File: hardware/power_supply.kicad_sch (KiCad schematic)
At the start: 13 parts, among them U103 K78L15-1000R3, U105 AMS1117-5, U106 AMS1117-3.3

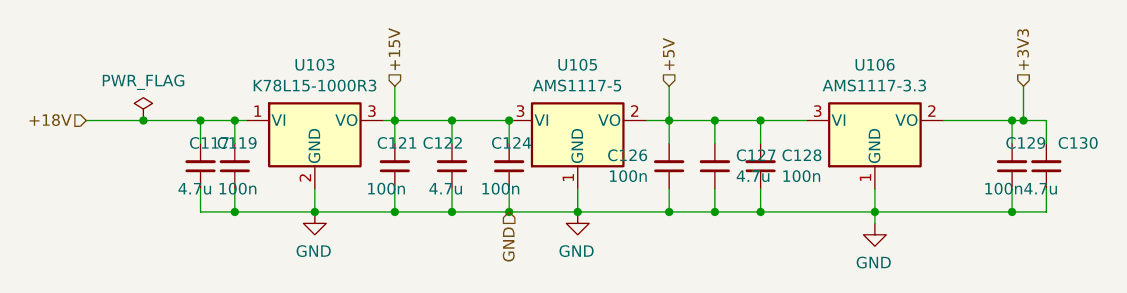
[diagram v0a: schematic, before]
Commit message: Atualização analog
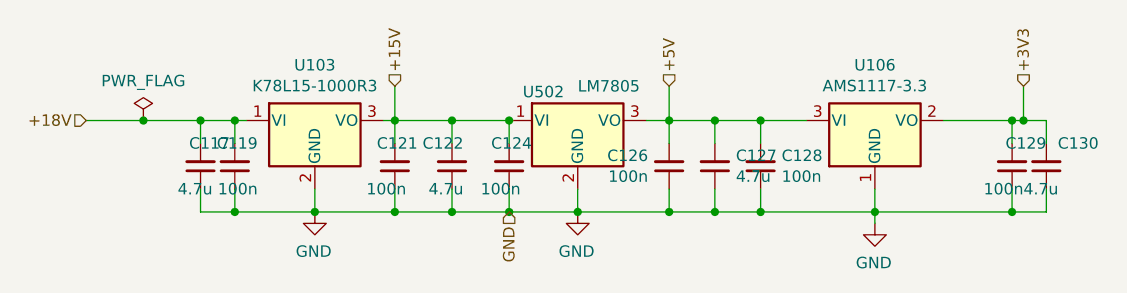
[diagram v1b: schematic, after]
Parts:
- removed U105: AMS1117-5, Package_TO_SOT_SMD:SOT-223-3_TabPin2, symbol Regulator_Linear:AP1117-15
- added U502: LM7805, KicadZeniteSolarLibrary18:TO-220-3_Horizontal_TabDown_SMD, symbol Regulator_Linear:LM7805_TO220
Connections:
- net +15V: now also U502.1 (VI)
- net +5V: now also U502.3 (VO)
- net GND: now also U502.2 (GND)
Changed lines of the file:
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@@
-	)
-	(junction
-		(at 138.43 64.77)
-		(diameter 0)
-		(color 0 0 0 0)
 	)
 	(junction
@@
 	(junction
 		(at 146.05 74.93)
+		(diameter 0)
+		(color 0 0 0 0)
+	)
+	(junction
+		(at 138.43 64.77)
 		(diameter 0)
 		(color 0 0 0 0)
@@
 	)
 	(symbol
+		(lib_id "Regulator_Linear:LM7805_TO220")
+		(at 146.05 64.77 0)
+		(unit 1)
+		(exclude_from_sim no)
+		(in_bom yes)
+		(on_board yes)
+		(dnp no)
+		(property "Reference" "U502"
+			(at 142.24 61.595 0)
+			(effects
+				(font
+					(size 1.27 1.27)
+				)
+			)
+		)
+		(property "Value" "LM7805"
+			(at 146.05 60.96 0)
+			(effects
+				(font
+					(size 1.27 1.27)
+				)
+				(justify left)
+			)
+		)
+		(property "Footprint" "KicadZeniteSolarLibrary18:TO-220-3_Horizontal_TabDown_SMD"
+			(at 146.05 59.055 0)
+			(effects
+				(font
+					(size 1.27 1.27)
+					(italic yes)
+				)
+				(hide yes)
+			)
+		)
+		(property "Datasheet" "https://www.sparkfun.com/datasheets/Components/LM7805.pdf"
+			(at 146.05 66.04 0)
+			(effects
+				(font
+					(size 1.27 1.27)
+				)
+				(hide yes)
+			)
+		)
+		(property "Description" ""
+			(at 146.05 64.77 0)
+			(effects
+				(font
+					(size 1.27 1.27)
+				)
+			)
+		)
+		(pin "1"
+		)
+		(pin "2"
+		)
+		(pin "3"
+		)
+		(instances
+			(project "MSG25"
+				(path "/65407f14-222c-4907-8176-906911332438/ba43f04b-a2b5-4499-bfc6-a32c11f6989d"
+					(reference "U502")
+					(unit 1)
+				)
+			)
+		)
+	)
+	(symbol
 		(lib_id "Device:C_Small")
 		(at 161.29 69.85 180)
@@
 					(unit 1)
 				)
-			)
-		)
-	)
-	(symbol
-		(lib_id "Regulator_Linear:AP1117-15")
-		(at 146.05 64.77 0)
-		(unit 1)
-		(exclude_from_sim no)
-		(in_bom yes)
-		(on_board yes)
-		(dnp no)
-		(property "Reference" "U105"
-			(at 146.05 58.6232 0)
-			(effects
-				(font
-					(size 1.27 1.27)
-				)
-			)
-		)
-		(property "Value" "AMS1117-5"
-			(at 146.05 60.9346 0)
-			(effects
-				(font
-					(size 1.27 1.27)
-				)
-			)
-		)
-		(property "Footprint" "Package_TO_SOT_SMD:SOT-223-3_TabPin2"
-			(at 146.05 59.69 0)
-			(effects
-				(font
-					(size 1.27 1.27)
-				)
-				(hide yes)
-			)
-		)
-		(property "Datasheet" ""
-			(at 148.59 71.12 0)
-			(effects
-				(font
-					(size 1.27 1.27)
-				)
-				(hide yes)
-			)
-		)
-		(property "Description" ""
-			(at 146.05 64.77 0)
-			(effects
-				(font
-					(size 1.27 1.27)
-				)
-				(hide yes)
-			)
-		)
-		(pin "1"
-		)
-		(pin "2"
-		)
-		(pin "3"
-		)
-		(instances
-			(project "MSG25"
-				(path "/65407f14-222c-4907-8176-906911332438/ba43f04b-a2b5-4499-bfc6-a32c11f6989d"
-					(reference "U105")
-					(unit 1)
-				)

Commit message: Placa Finalizada para revisão
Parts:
- U103: footprint KicadZeniteSolarLibrary18:TO-220-3_Horizontal_Tabless_SMD -> Package_TO_SOT_THT:TO-220-3_Horizontal_TabDown
- U502: footprint KicadZeniteSolarLibrary18:TO-220-3_Horizontal_TabDown_SMD -> Package_TO_SOT_THT:TO-220-3_Horizontal_TabDown
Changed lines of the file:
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@@
 			)
 		)
-		(property "Footprint" "KicadZeniteSolarLibrary18:TO-220-3_Horizontal_TabDown_SMD"
+		(property "Footprint" "Package_TO_SOT_THT:TO-220-3_Horizontal_TabDown"
 			(at 146.05 59.055 0)
 			(effects
@@
 			)
 		)
-		(property "Footprint" "KicadZeniteSolarLibrary18:TO-220-3_Horizontal_Tabless_SMD"
+		(property "Footprint" "Package_TO_SOT_THT:TO-220-3_Horizontal_TabDown"
 			(at 116.84 59.055 0)
 			(effects
